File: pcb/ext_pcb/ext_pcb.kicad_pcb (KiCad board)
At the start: 2 copper layers, 78 x 37.5 mm, 19 parts, among them J1 SFW15R-2STE1LF, J2 Conn_01x04_Pin, J3 Conn_01x04_Pin, J4 SJ2-3574A-SMT-TR, J5 Conn_02x07_Counter_Clockwise

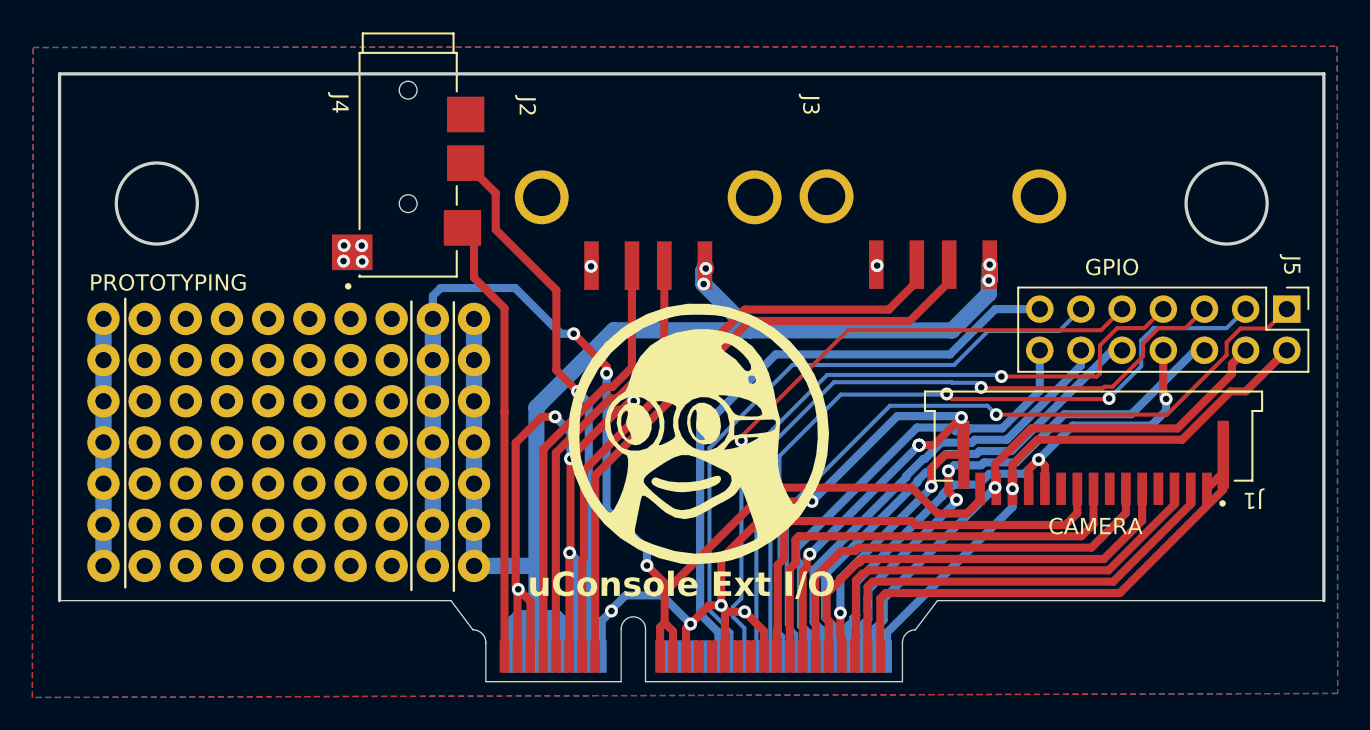
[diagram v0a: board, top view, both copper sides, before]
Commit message: REV: A
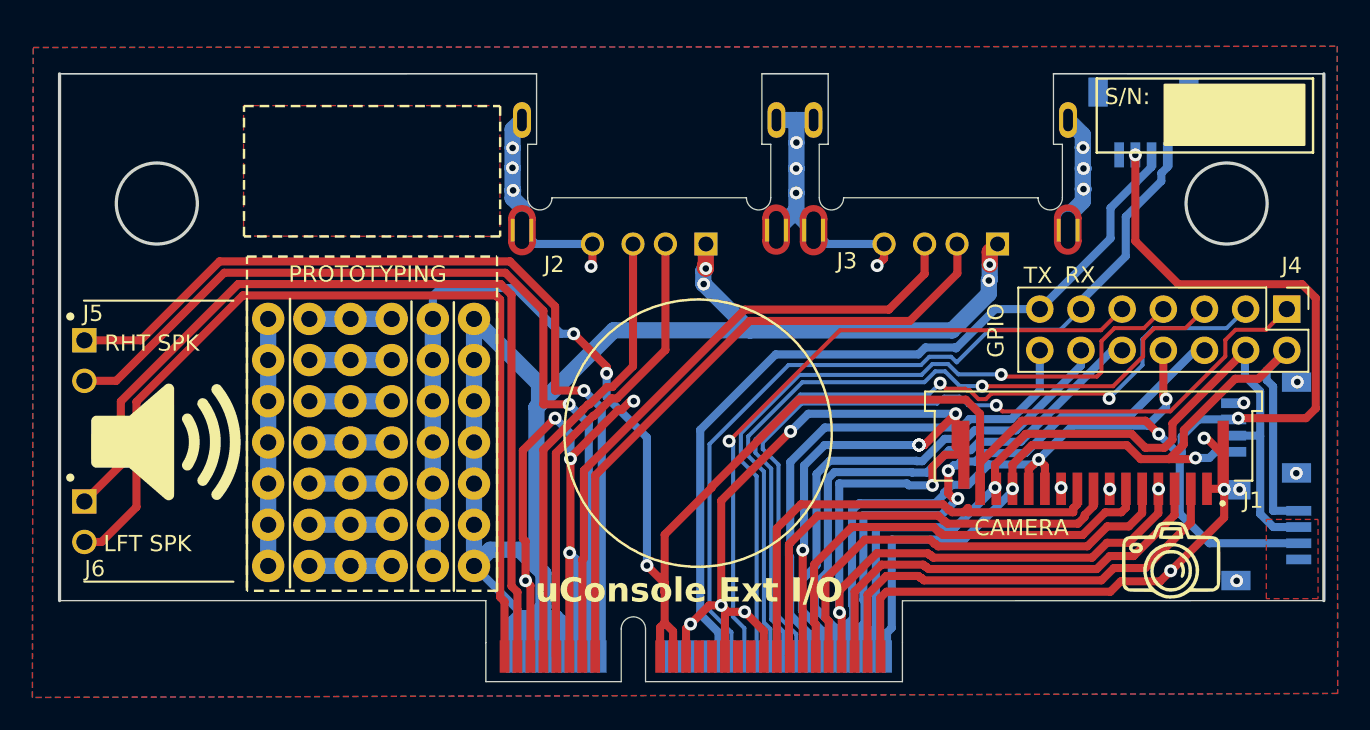
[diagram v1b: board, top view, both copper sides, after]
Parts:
- removed the J4 at (130.6, 73.7)
- removed the REF** at (114.3, 83.8)
- removed the REF** at (121.9, 83.8)
- removed the REF** at (116.8, 83.8)
- removed the REF** at (119.4, 83.8)
- added G***: LOGO, LOGO, F.Cu at (115.5, 91.3)
- added G***: LOGO, LOGO, F.Cu at (128.3, 74.7)
- added G***: LOGO, LOGO, F.Cu at (177.6, 98.5)
- added G***: LOGO, LOGO, B.Cu at (183.8, 71.3)
- added G***: LOGO, LOGO, B.Cu at (127.0, 78.2)
- added G***: LOGO, LOGO, B.Cu at (178.2, 93.9)
- added J5: S2B-XH-A(LF)(SN), 1_project:JST_S2B-XH-A(LF)(SN), F.Cu at (110.6, 86.4)
- added J6: S2B-XH-A(LF)(SN), 1_project:JST_S2B-XH-A(LF)(SN), F.Cu at (110.6, 96.3)
- added J7: SM04B-SRSS-TB(LF)(SN), 1_project:JST_SM04B-SRSS-TB(LF)(SN), B.Cu at (185.5, 97.2)
- added J8: SM04B-SRSS-TB(LF)(SN), 1_project:JST_SM04B-SRSS-TB(LF)(SN), B.Cu at (181.5, 90.5)
- added J9: SM04B-SRSS-TB(LF)(SN), 1_project:JST_SM04B-SRSS-TB(LF)(SN), B.Cu at (175.9, 73.7)
- J2, J3: value Conn_01x04_Pin -> GSB12J21C1EU; footprint 1_project:USB_TYPE_A -> 1_project:GSB12J21C1EU; moved to B.Cu
- moved REF** 10.2 mm to (121.9, 83.8)
- moved J2 7.62 mm to (145.4, 68.7), turned to 0 degrees
- moved J3 7.58 mm to (163.4, 68.7), turned to 0 degrees
- moved G*** 1.85 mm to (154.9, 86.4)
- renumbered J5 to J4
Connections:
- net /GPIO32_CM14 renamed /GPIO32_CM14_TX0
- net /GPIO33_CM15 renamed /GPIO33_CM15_RX0
- J1 pad 1: /GND -> GND
- J1 pad 10: /GND -> GND
- J1 pad 4: /GND -> GND
- J1 pad 7: /GND -> GND
- J1 pad S1: /GND -> GND
- J1 pad S2: /GND -> GND
- J2 pad 4: /GND -> GND
- J3 pad 4: /GND -> GND
- P1 pad 11: /GND -> GND
- P1 pad 12: /GND -> GND
- P1 pad 16: /GND -> /SPK_RN
- P1 pad 21: /GND -> GND
- P1 pad 27: /GND -> GND
- P1 pad 3: /GND -> /SPK_LN
- P1 pad 33: /GND -> GND
- P1 pad 39: /GND -> GND
- P1 pad 45: /GND -> GND
- P1 pad 5: /GND -> GND
- P1 pad 51: /GND -> GND
- REF** pad 1: /GND -> GND
- REF** pad 2: /GND -> GND
- REF** pad 3: /GND -> GND
- REF** pad 4: /GND -> GND
- REF** pad 5: /GND -> GND
- REF** pad 6: /GND -> GND
- REF** pad 7: /GND -> GND
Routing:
- net GND: track 0.00 -> 238.2 mm, vias 0 -> 38
- net /GND: track 176.6 -> 0.00 mm, vias 23 -> 0
- net /3.3V: track 75.2 -> 143.7 mm, vias 3 -> 6
- net /SPK_LN: track 0.00 -> 56.9 mm
- net /SPK_RN: track 0.00 -> 56.0 mm, vias 0 -> 1
- net (no net): track 0.00 -> 35.6 mm
- net /SPK_LP: track 27.5 -> 58.0 mm
- net /SPK_RP: track 33.6 -> 55.7 mm
- net /GPIO45_CM_SCL0: track 34.9 -> 55.1 mm, vias 1 -> 2
- net /GPIO44_CM_SDA0: track 33.7 -> 52.3 mm
- net /5V: track 85.7 -> 101.1 mm
- net /GPIO32_CM14_TX0: track 38.5 -> 50.9 mm
- net /GPIO33_CM15_RX0: track 39.9 -> 52.1 mm
- net /GPIO38_CM6: track 46.2 -> 51.1 mm
- net /GPIO40_CM16: track 28.3 -> 32.2 mm
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- added copper zone on B.Cu, net GND
- added copper zone on F.Cu, net GND
- removed copper zone on B.Cu, net /GND
- removed copper zone on F.Cu, net /GND
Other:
- outline, holes or cut-outs redrawn
- board text added: "LFT SPK"
- board text added: "P/N: 57B-20230703-001 REV: A, 2023-07-07"
- board text added: "RHT SPK"
- board text added: "RT3G"
- board text added: "RX"
- board text added: "TX"
- board text removed: "P/N: 57B-20230703-001 REV: -, 2023-07-03"
